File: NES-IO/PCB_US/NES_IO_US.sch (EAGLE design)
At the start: 62 parts, among them IC1 74HC125D, J1.1 MY_JUMPER, J1.2 MY_JUMPER, J2.2 10k, J6 MY_JUMPER, J7 MY_JUMPER

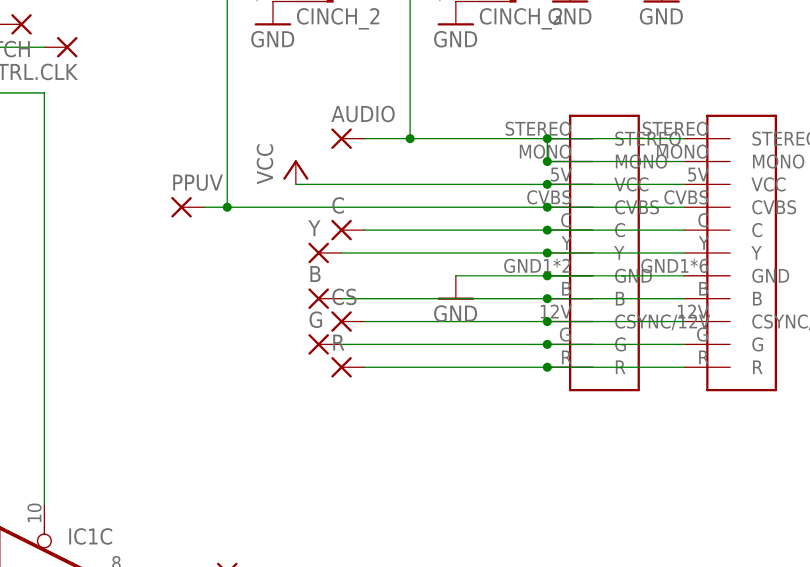
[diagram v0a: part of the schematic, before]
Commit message: Update PCB files
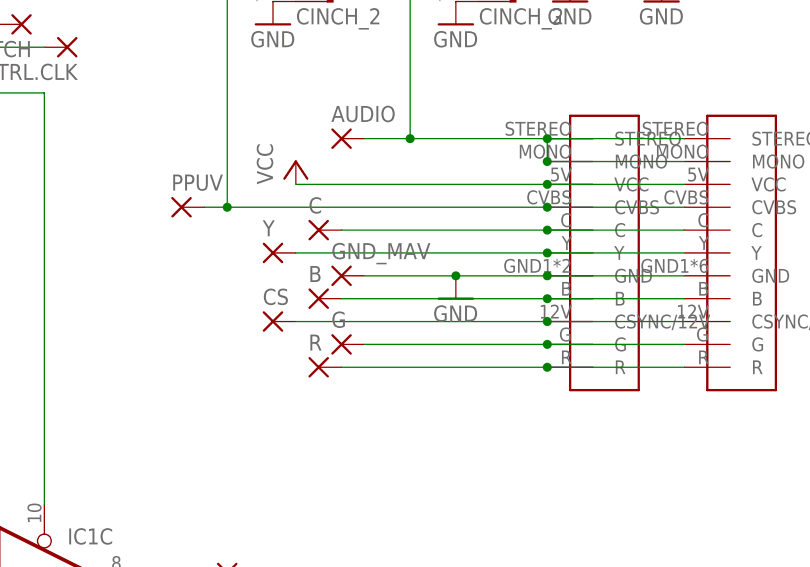
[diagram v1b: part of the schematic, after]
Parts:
- added GND_MAV: (no value), wirepad:SMD2
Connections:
- net GND: now also GND_MAV.P
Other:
- moved on the sheet: C, CS, G, R, Y
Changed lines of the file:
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@@
 <part name="GND10" library="wirepad" deviceset="SMD5" device=""/>
 <part name="GND11" library="supply1" deviceset="GND" device=""/>
+<part name="GND_MAV" library="wirepad" deviceset="SMD2" device=""/>
 <part name="U$5" library="snes_div" deviceset="PIC16F630_SIMPLE" device=""/>
 <part name="P+4" library="supply1" deviceset="VCC" device=""/>
@@
 <part name="GND16" library="supply1" deviceset="GND" device=""/>
 <part name="GND29" library="supply1" deviceset="GND" device=""/>
+<part name="C" library="wirepad" deviceset="SMD2" device=""/>
 <part name="Y" library="wirepad" deviceset="SMD2" device=""/>
-<part name="C" library="wirepad" deviceset="SMD2" device=""/>
 </parts>
 <sheets>
@@
 <instance part="AUDIO" gate="1" x="22.86" y="99.06"/>
 <instance part="PPUV" gate="1" x="5.08" y="91.44"/>
-<instance part="CS" gate="1" x="22.86" y="78.74"/>
-<instance part="R" gate="1" x="22.86" y="73.66"/>
-<instance part="G" gate="1" x="20.32" y="76.2"/>
+<instance part="CS" gate="1" x="15.24" y="78.74"/>
+<instance part="R" gate="1" x="20.32" y="73.66"/>
+<instance part="G" gate="1" x="22.86" y="76.2"/>
 <instance part="B" gate="1" x="20.32" y="81.28"/>
 <instance part="GND" gate="1" x="104.14" y="88.9"/>
 <instance part="GND10" gate="1" x="104.14" y="86.36"/>
 <instance part="GND11" gate="1" x="109.22" y="81.28"/>
+<instance part="GND_MAV" gate="1" x="22.86" y="83.82"/>
 <instance part="U$5" gate="G$1" x="-58.42" y="106.68"/>
 <instance part="U$5" gate="G$2" x="-58.42" y="132.08" rot="R90"/>
@@
 <instance part="GND16" gate="1" x="15.24" y="111.76"/>
 <instance part="GND29" gate="1" x="35.56" y="111.76"/>
-<instance part="Y" gate="1" x="20.32" y="86.36"/>
-<instance part="C" gate="1" x="22.86" y="88.9"/>
+<instance part="C" gate="1" x="20.32" y="88.9"/>
+<instance part="Y" gate="1" x="15.24" y="86.36"/>
 </instances>
 <busses>
@@
 <pinref part="GND4" gate="1" pin="GND"/>
 <wire x1="60.96" y1="83.82" x2="45.72" y2="83.82" width="0.1524" layer="91"/>
+<pinref part="GND_MAV" gate="1" pin="P"/>
 <wire x1="45.72" y1="83.82" x2="35.56" y2="83.82" width="0.1524" layer="91"/>
+<wire x1="35.56" y1="83.82" x2="25.4" y2="83.82" width="0.1524" layer="91"/>
+<junction x="35.56" y="83.82"/>
 <pinref part="U$20" gate="G$1" pin="GND"/>
 <junction x="45.72" y="83.82"/>
@@
 </segment>
 </net>
-<net name="N$7" class="0">
-<segment>
-<pinref part="CS" gate="1" pin="P"/>
-<pinref part="U$19" gate="G$1" pin="CSYNC/12V"/>
-<wire x1="60.96" y1="78.74" x2="45.72" y2="78.74" width="0.1524" layer="91"/>
-<pinref part="U$20" gate="G$1" pin="CSYNC/12V"/>
-<junction x="45.72" y="78.74"/>
-<wire x1="25.4" y1="78.74" x2="45.72" y2="78.74" width="0.1524" layer="91"/>
-</segment>
-</net>
 <net name="N$8" class="0">
 <segment>
@@
 <wire x1="60.96" y1="76.2" x2="45.72" y2="76.2" width="0.1524" layer="91"/>
 <pinref part="U$20" gate="G$1" pin="G"/>
-<wire x1="45.72" y1="76.2" x2="22.86" y2="76.2" width="0.1524" layer="91"/>
+<wire x1="45.72" y1="76.2" x2="25.4" y2="76.2" width="0.1524" layer="91"/>
 <junction x="45.72" y="76.2"/>
 <pinref part="U$19" gate="G$1" pin="G"/>
@@
 <wire x1="60.96" y1="73.66" x2="45.72" y2="73.66" width="0.1524" layer="91"/>
 <pinref part="U$20" gate="G$1" pin="R"/>
-<wire x1="45.72" y1="73.66" x2="25.4" y2="73.66" width="0.1524" layer="91"/>
+<wire x1="45.72" y1="73.66" x2="22.86" y2="73.66" width="0.1524" layer="91"/>
 <junction x="45.72" y="73.66"/>
 <pinref part="U$19" gate="G$1" pin="R"/>
@@
 </segment>
 </net>
-<net name="N$11" class="0">
-<segment>
-<pinref part="3" gate="1" pin="P"/>
-<pinref part="IC1" gate="C" pin="O"/>
-<wire x1="7.62" y1="50.8" x2="0" y2="50.8" width="0.1524" layer="91"/>
-</segment>
-</net>
-<net name="N$27" class="0">
-<segment>
-<pinref part="1" gate="1" pin="P"/>
-<pinref part="IC1" gate="A" pin="O"/>
-<wire x1="7.62" y1="30.48" x2="-27.94" y2="30.48" width="0.1524" layer="91"/>
-</segment>
-</net>
-<net name="N$29" class="0">
-<segment>
+<net name="N$30" class="0">
+<segment>
+<wire x1="10.16" y1="91.44" x2="45.72" y2="91.44" width="0.1524" layer="91"/>
+<wire x1="45.72" y1="91.44" x2="60.96" y2="91.44" width="0.1524" layer="91"/>
+<pinref part="U$20" gate="G$1" pin="CVBS"/>
+<junction x="45.72" y="91.44"/>
+<pinref part="U$19" gate="G$1" pin="CVBS"/>
 <pinref part="PPUV" gate="1" pin="P"/>
 <wire x1="10.16" y1="91.44" x2="7.62" y2="91.44" width="0.1524" layer="91"/>
@@
 <wire x1="15.24" y1="116.84" x2="10.16" y2="116.84" width="0.1524" layer="91"/>
 <wire x1="10.16" y1="116.84" x2="10.16" y2="91.44" width="0.1524" layer="91"/>
-<wire x1="10.16" y1="91.44" x2="45.72" y2="91.44" width="0.1524" layer="91"/>
-<wire x1="45.72" y1="91.44" x2="60.96" y2="91.44" width="0.1524" layer="91"/>
-<pinref part="U$20" gate="G$1" pin="CVBS"/>
-<junction x="45.72" y="91.44"/>
-<pinref part="U$19" gate="G$1" pin="CVBS"/>
+</segment>
+</net>
+<net name="N$11" class="0">
+<segment>
+<pinref part="3" gate="1" pin="P"/>
+<pinref part="IC1" gate="C" pin="O"/>
+<wire x1="7.62" y1="50.8" x2="0" y2="50.8" width="0.1524" layer="91"/>
+</segment>
+</net>
+<net name="N$27" class="0">
+<segment>
+<pinref part="1" gate="1" pin="P"/>
+<pinref part="IC1" gate="A" pin="O"/>
+<wire x1="7.62" y1="30.48" x2="-27.94" y2="30.48" width="0.1524" layer="91"/>
 </segment>
 </net>
@@
 </segment>
 </net>
+<net name="N$1" class="0">
+<segment>
+<pinref part="U$19" gate="G$1" pin="CSYNC/12V"/>
+<wire x1="60.96" y1="78.74" x2="45.72" y2="78.74" width="0.1524" layer="91"/>
+<pinref part="U$20" gate="G$1" pin="CSYNC/12V"/>
+<pinref part="CS" gate="1" pin="P"/>
+<wire x1="45.72" y1="78.74" x2="17.78" y2="78.74" width="0.1524" layer="91"/>
+<junction x="45.72" y="78.74"/>
+</segment>
+</net>
 <net name="N$2" class="0">
 <segment>
@@
 <pinref part="U$20" gate="G$1" pin="Y"/>
 <pinref part="Y" gate="1" pin="P"/>
-<wire x1="45.72" y1="86.36" x2="22.86" y2="86.36" width="0.1524" layer="91"/>
+<wire x1="17.78" y1="86.36" x2="45.72" y2="86.36" width="0.1524" layer="91"/>
 <junction x="45.72" y="86.36"/>
 </segment>
 </net>
-<net name="N$1" class="0">
-<segment>
+<net name="N$3" class="0">
+<segment>
+<pinref part="U$20" gate="G$1" pin="C"/>
 <pinref part="C" gate="1" pin="P"/>
-<pinref part="U$20" gate="G$1" pin="C"/>
-<wire x1="25.4" y1="88.9" x2="45.72" y2="88.9" width="0.1524" layer="91"/>
+<wire x1="45.72" y1="88.9" x2="22.86" y2="88.9" width="0.1524" layer="91"/>
 <pinref part="U$19" gate="G$1" pin="C"/>
 <wire x1="60.96" y1="88.9" x2="45.72" y2="88.9" width="0.1524" layer="91"/>
